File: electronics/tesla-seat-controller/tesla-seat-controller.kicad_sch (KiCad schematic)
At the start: 40 parts, among them J1 12V In, J2 SWD, J3 USB_C_Receptacle, SW1 SW_Push, U1 AP63203WU, U2 RP2354, Y1 ABM8-272-T3

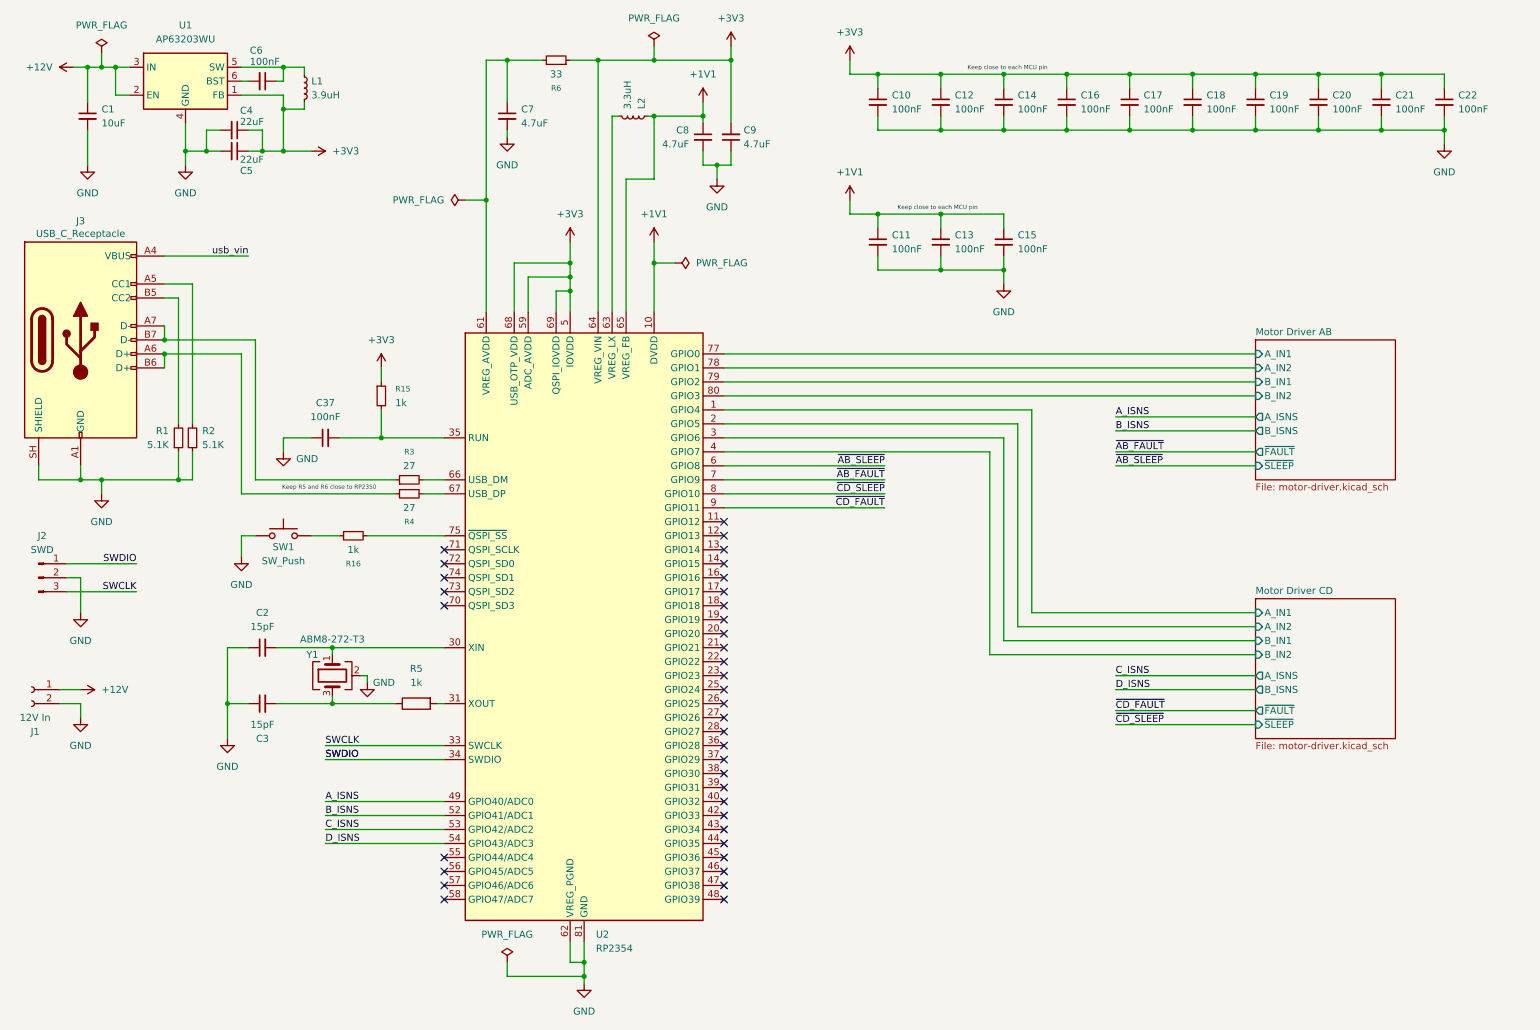
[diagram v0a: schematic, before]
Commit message: Finish out protection + fan
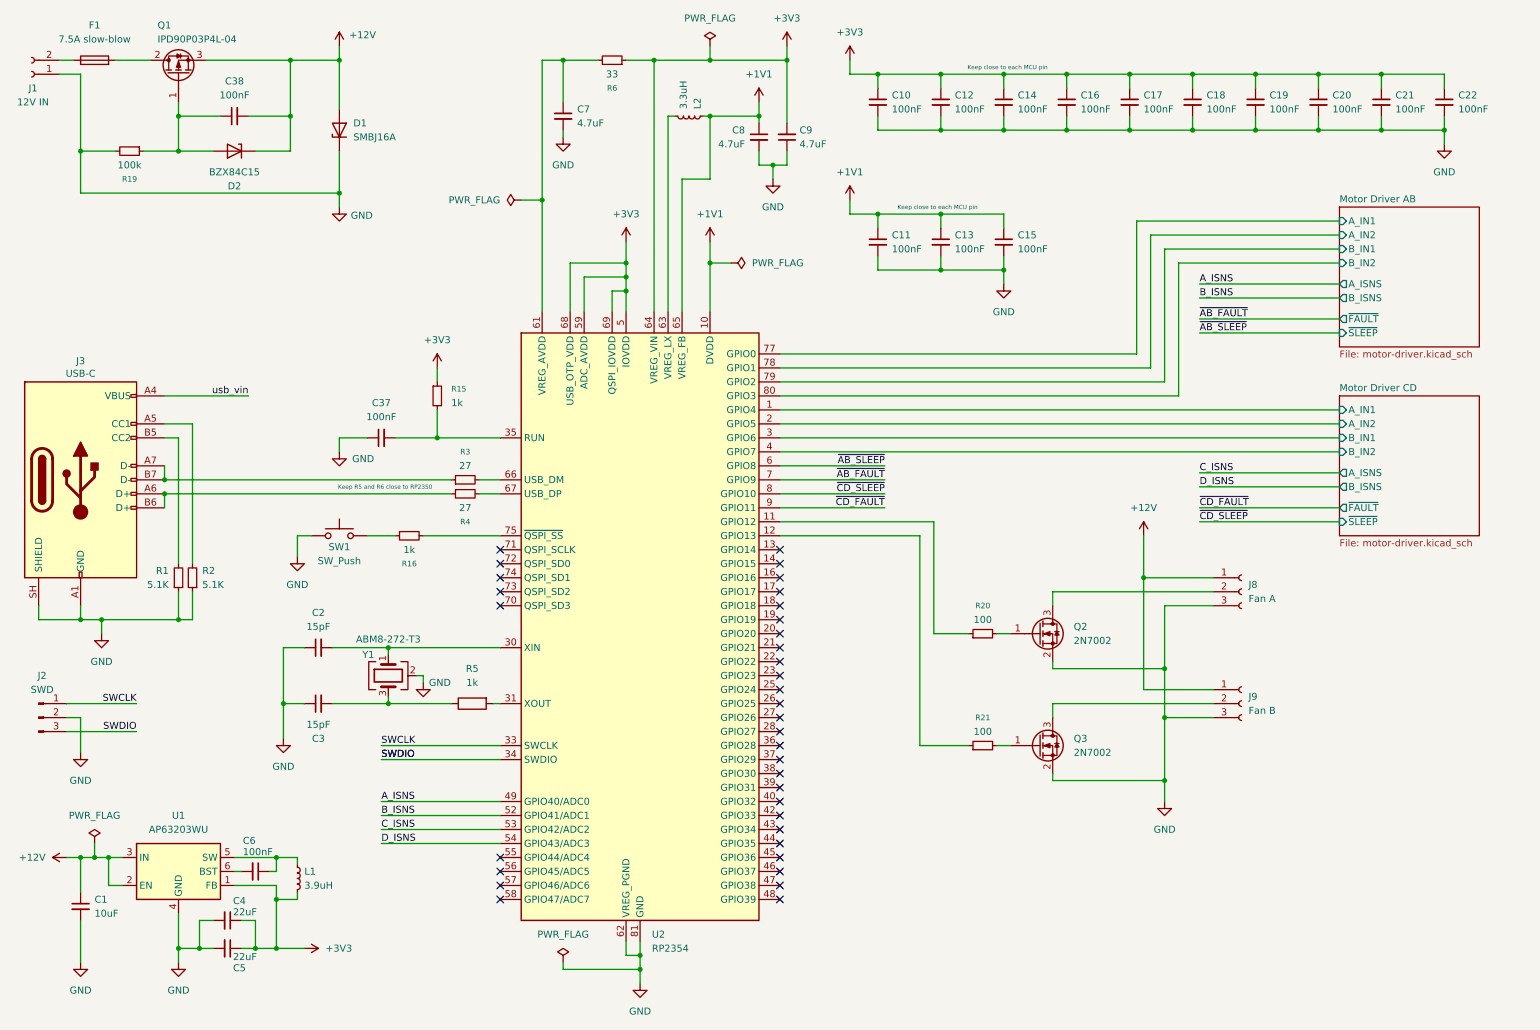
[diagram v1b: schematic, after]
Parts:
- added C38: 100nF, symbol Device:C_Small
- added D1: SMBJ16A, symbol Device:D_Zener
- added D2: BZX84C15, symbol Device:D_Zener
- added F1: 7.5A slow-blow, symbol Device:Fuse
- added J8: Fan A, symbol Connector:Conn_01x03_Socket
- added J9: Fan B, symbol Connector:Conn_01x03_Socket
- added Q1: IPD90P03P4L-04, symbol Transistor_FET:Q_PMOS_GDS
- added Q2, Q3: 2N7002, Package_TO_SOT_SMD:SOT-23, symbol Transistor_FET:2N7002
- added R19: 100k, symbol Device:R_Small
- added R20, R21: 100, symbol Device:R_Small
- J1: value 12V In -> 12V IN
- J3: value USB_C_Receptacle -> USB-C
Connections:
- net +12V: now also C38.2, D1.2 (A), D2.1 (K), J8.1 (Pin_1), J9.1 (Pin_1), Q1.3 (S); no longer J1.1 (Pin_1)
- net GND: now also J1.1 (Pin_1), D1.1 (K), J8.3 (Pin_3), J9.3 (Pin_3), Q2.2 (S), Q3.2 (S), R19.2; no longer J1.2 (Pin_2)
- net SWCLK: now also J2.1 (Pin_1); no longer J2.3 (Pin_3)
- net SWDIO: now also J2.3 (Pin_3); no longer J2.1 (Pin_1)
- net at U2.11 (GPIO12): now also R20.1
- net at U2.12 (GPIO13): now also R21.1
- new net: Q2.1 (G), R20.2
- new net: C38.1, D2.2 (A), Q1.1 (G), R19.1
- new net: Q3.1 (G), R21.2
- new net: F1.2, Q1.2 (D)
- new net: J8.2 (Pin_2), Q2.3 (D)
- new net: F1.1, J1.2 (Pin_2)
- new net: J9.2 (Pin_2), Q3.3 (D)
- no-connect marks 37 -> 35
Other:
- moved on the sheet: C1, C2, C3, C37, C4, C5, C6, C7, C8, C9, J1, J2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
